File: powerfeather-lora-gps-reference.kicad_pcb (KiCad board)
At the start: 2 copper layers, 23 x 58 mm, 18 parts, among them J1 Conn_01x05, J11 Conn_01x04, J2 Conn_01x02, J3 Conn_01x04, J4 Conn_01x02, J5 Conn_01x02, J6 Conn_01x04, J7 Conn_01x04, J8 Conn_01x03, J9 Conn_01x03, U2 Lora126x, Y1 32.768 kHz

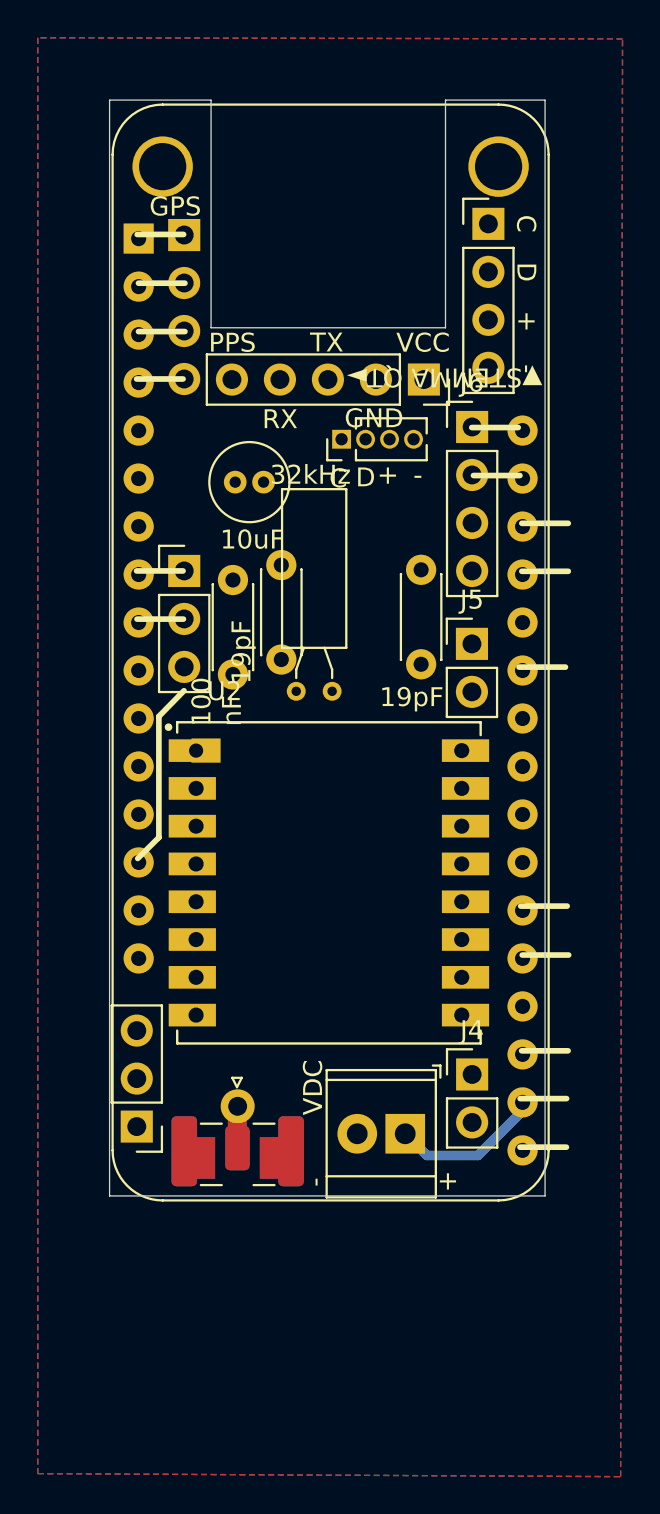
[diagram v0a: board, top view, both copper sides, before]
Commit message: Rearrange rough layout again
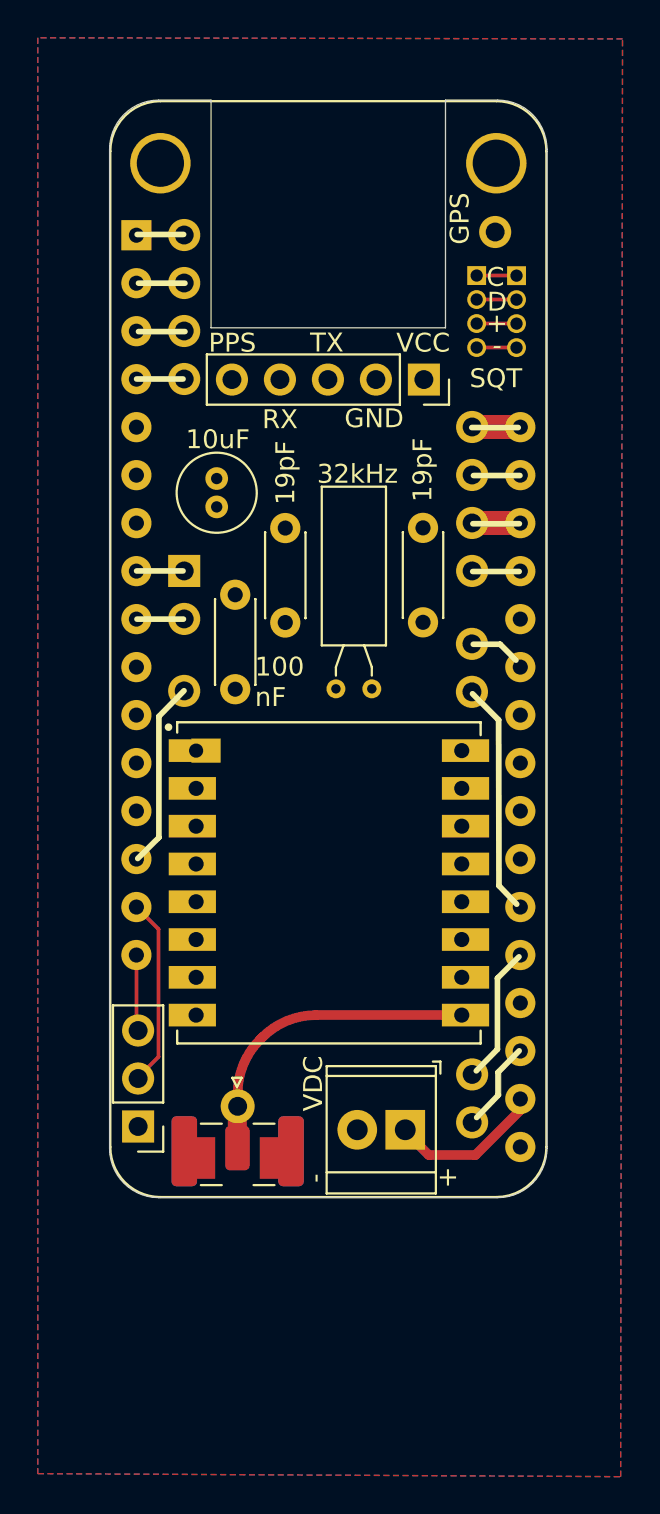
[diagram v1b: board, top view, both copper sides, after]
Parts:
- added J10: Conn_01x01, Connector_PinHeader_2.54mm:PinHeader_1x01_P2.54mm_Vertical, F.Cu at (140.0, 76.5)
- J3: footprint Connector_PinHeader_2.54mm:PinHeader_1x04_P2.54mm_Vertical -> Connector_PinHeader_1.27mm:PinHeader_1x04_P1.27mm_Vertical
- moved J7 12.7 mm to (141.1, 78.8), turned to 0 degrees
- moved J3 2.80 mm to (139.0, 78.8)
- moved C1 2.22 mm to (136.1, 97.1)
- moved Y1 2.10 mm to (133.4, 100.7)
- moved C2 1.97 mm to (128.8, 97.2)
- moved C4 1.64 mm to (125.2, 91.0), turned to 90 degrees
- moved C3 0.79 mm to (126.2, 95.7)
- moved A1 0.22 mm to (121.0, 76.7)
- moved J2 0.21 mm to (135.2, 124.0)
- moved J9 0.07 mm to (121.1, 123.8)
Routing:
- net Net-(AE1-A): track 0.00 -> 14.9 mm
- net /SCL: track 0.00 -> 12.5 mm
- net /RXD0: track 0.00 -> 10.0 mm
- net /SDA: track 0.00 -> 7.38 mm
- net /D7: track 0.00 -> 4.84 mm
- net /TXD0: track 0.00 -> 4.01 mm
- net /D11: track 0.00 -> 3.19 mm
- net VS: track 0.00 -> 2.55 mm
- net /D13: track 0.00 -> 2.55 mm
- net +BATT: track 0.00 -> 2.55 mm
- net /EN: track 0.00 -> 2.55 mm
- net /SCL1: track 0.00 -> 2.11 mm
- net GND: track 0.00 -> 2.11 mm
- net /SDA1: track 0.00 -> 2.11 mm
- net +3.3VP: track 0.00 -> 2.11 mm
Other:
- board size 23 x 58 mm -> 23.1 x 58.1 mm
